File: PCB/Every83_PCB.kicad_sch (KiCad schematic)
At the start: 31 parts, among them J1 781710004, J3 SM03B-SRSS-TB, J4 SM03B-SRSS-TB, Q3 DMG2305, SW101 KMR2, SW102 KMR2, U1 Core52840, U2 AP2112(3.3V), U3 MCP73831T-2ACI/OT, X3 JSTPH

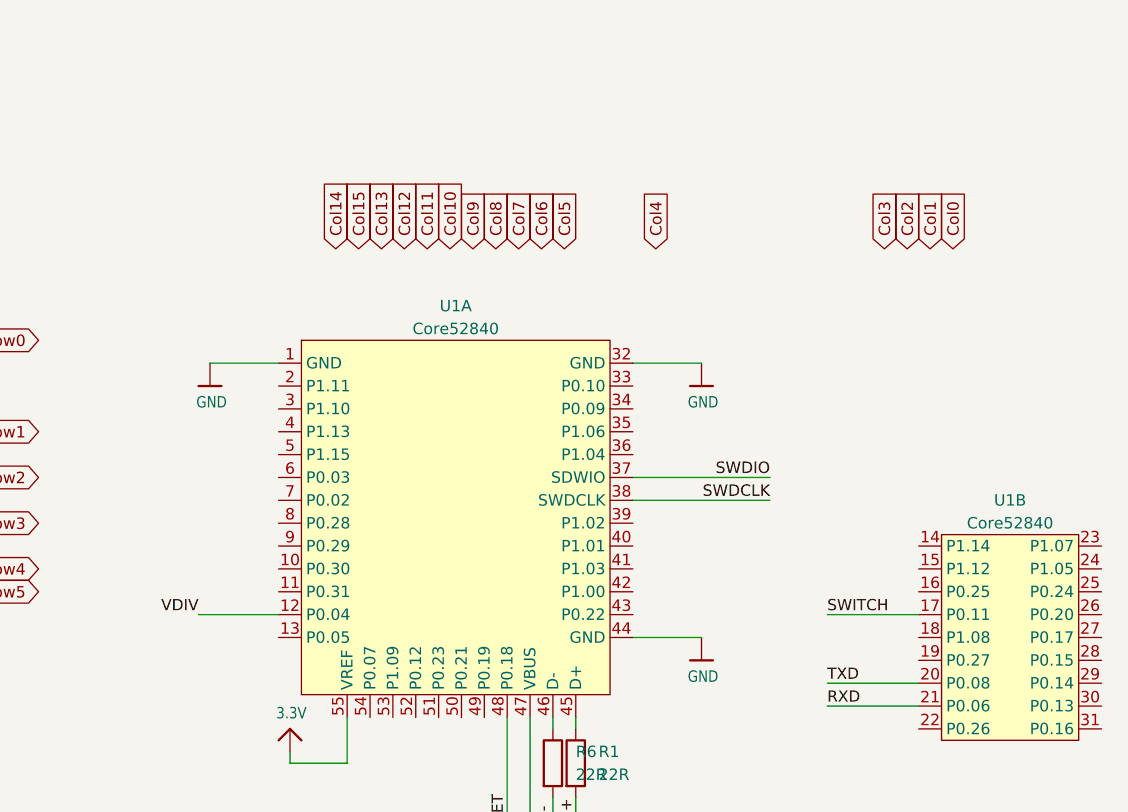
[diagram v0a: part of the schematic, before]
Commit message: More work done
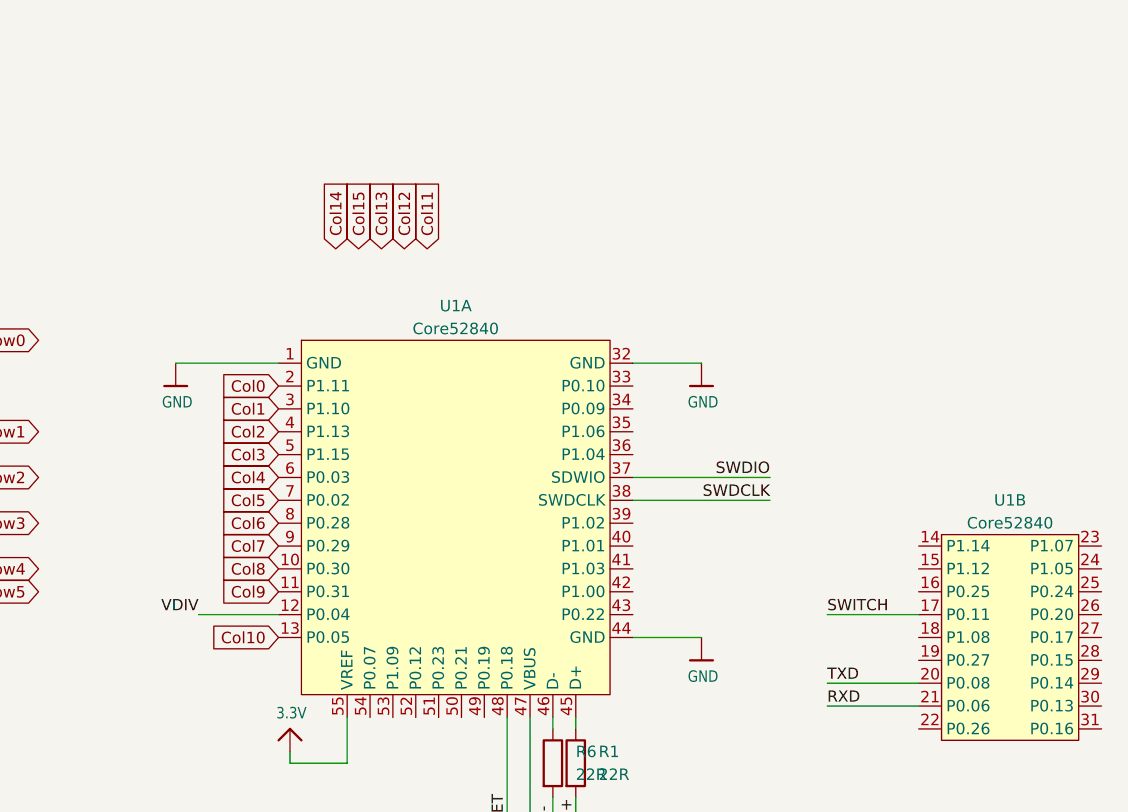
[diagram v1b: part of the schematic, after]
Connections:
- net Col0: now also U1.2 (P1.11)
- net Col1: now also U1.3 (P1.10)
- net Col10: now also U1.13 (P0.05)
- net Col2: now also U1.4 (P1.13)
- net Col3: now also U1.5 (P1.15)
- net Col4: now also U1.6 (P0.03)
- net Col5: now also U1.7 (P0.02)
- net Col6: now also U1.8 (P0.28)
- net Col7: now also U1.9 (P0.29)
- net Col8: now also U1.10 (P0.30)
- net Col9: now also U1.11 (P0.31)
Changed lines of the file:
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@@
 	(wire
 		(pts
-			(xy 120.65 81.28) (xy 128.27 81.28)
+			(xy 116.84 81.28) (xy 128.27 81.28)
 		)
 		(stroke
@@
 	(global_label "Col10"
 		(shape input)
-		(at 147.32 68.58 90)
+		(at 128.27 111.76 180)
 		(fields_autoplaced yes)
 		(effects
@@
 				(size 1.27 1.27)
 			)
-			(justify left)
+			(justify right)
 		)
 		(property "Intersheetrefs" "${INTERSHEET_REFS}"
-			(at 147.32 60.171 90)
+			(at 119.7816 111.76 0)
 			(effects
 				(font
 					(size 1.27 1.27)
 				)
-				(justify left)
+				(justify right)
 				(hide yes)
 			)
@@
 	(global_label "Col8"
 		(shape input)
-		(at 152.4 68.58 90)
+		(at 128.27 104.14 180)
 		(fields_autoplaced yes)
 		(effects
@@
 				(size 1.27 1.27)
 			)
-			(justify left)
+			(justify right)
 		)
 		(property "Intersheetrefs" "${INTERSHEET_REFS}"
-			(at 152.4 61.3011 90)
+			(at 120.9911 104.14 0)
 			(effects
 				(font
 					(size 1.27 1.27)
 				)
-				(justify left)
+				(justify right)
 				(hide yes)
 			)
@@
 	(global_label "Col5"
 		(shape input)
-		(at 160.02 68.58 90)
+		(at 128.27 96.52 180)
 		(fields_autoplaced yes)
 		(effects
@@
 				(size 1.27 1.27)
 			)
-			(justify left)
+			(justify right)
 		)
 		(property "Intersheetrefs" "${INTERSHEET_REFS}"
-			(at 160.02 61.3011 90)
+			(at 120.9911 96.52 0)
 			(effects
 				(font
 					(size 1.27 1.27)
 				)
-				(justify left)
+				(justify right)
 				(hide yes)
 			)
@@
 	(global_label "Col7"
 		(shape input)
-		(at 154.94 68.58 90)
+		(at 128.27 101.6 180)
 		(fields_autoplaced yes)
 		(effects
@@
 				(size 1.27 1.27)
 			)
-			(justify left)
+			(justify right)
 		)
 		(property "Intersheetrefs" "${INTERSHEET_REFS}"
-			(at 154.94 61.3011 90)
+			(at 120.9911 101.6 0)
 			(effects
 				(font
 					(size 1.27 1.27)
 				)
-				(justify left)
+				(justify right)
 				(hide yes)
 			)
@@
 	(global_label "Col9"
 		(shape input)
-		(at 149.86 68.58 90)
+		(at 128.27 106.68 180)
 		(fields_autoplaced yes)
 		(effects
@@
 				(size 1.27 1.27)
 			)
-			(justify left)
+			(justify right)
 		)
 		(property "Intersheetrefs" "${INTERSHEET_REFS}"
-			(at 149.86 61.3805 90)
+			(at 120.9911 106.68 0)
 			(effects
 				(font
 					(size 1.27 1.27)
 				)
-				(justify left)
+				(justify right)
 				(hide yes)
 			)
@@
 	(global_label "Col6"
 		(shape input)
-		(at 157.48 68.58 90)
+		(at 128.27 99.06 180)
 		(fields_autoplaced yes)
 		(effects
@@
 				(size 1.27 1.27)
 			)
-			(justify left)
+			(justify right)
 		)
 		(property "Intersheetrefs" "${INTERSHEET_REFS}"
-			(at 157.48 61.3011 90)
+			(at 120.9911 99.06 0)
 			(effects
 				(font
 					(size 1.27 1.27)
 				)
-				(justify left)
+				(justify right)
 				(hide yes)
 			)
@@
 	(global_label "Col2"
 		(shape input)
-		(at 198.12 68.58 90)
+		(at 128.27 88.9 180)
 		(fields_autoplaced yes)
 		(effects
@@
 				(size 1.27 1.27)
 			)
-			(justify left)
+			(justify right)
 		)
 		(property "Intersheetrefs" "${INTERSHEET_REFS}"
-			(at 198.12 61.3011 90)
+			(at 120.9911 88.9 0)
 			(effects
 				(font
 					(size 1.27 1.27)
 				)
-				(justify left)
+				(justify right)
 				(hide yes)
 			)
@@
 	(global_label "Col3"
 		(shape input)
-		(at 195.58 68.58 90)
+		(at 128.27 91.44 180)
 		(fields_autoplaced yes)
 		(effects
@@
 				(size 1.27 1.27)
 			)
-			(justify left)
+			(justify right)
 		)
 		(property "Intersheetrefs" "${INTERSHEET_REFS}"
-			(at 195.58 61.3011 90)
+			(at 120.9911 91.44 0)
 			(effects
 				(font
 					(size 1.27 1.27)
 				)
-				(justify left)
+				(justify right)
 				(hide yes)
 			)
@@
 	(global_label "Col1"
 		(shape input)
-		(at 200.66 68.58 90)
+		(at 128.27 86.36 180)
 		(fields_autoplaced yes)
 		(effects
@@
 				(size 1.27 1.27)
 			)
-			(justify left)
+			(justify right)
 		)
 		(property "Intersheetrefs" "${INTERSHEET_REFS}"
-			(at 200.66 61.3011 90)
+			(at 120.9911 86.36 0)
 			(effects
 				(font
 					(size 1.27 1.27)
 				)
-				(justify left)
+				(justify right)
 				(hide yes)
 			)
@@
 	(global_label "Col0"
 		(shape input)
-		(at 203.2 68.58 90)
+		(at 128.27 83.82 180)
 		(fields_autoplaced yes)
 		(effects
@@
 				(size 1.27 1.27)
 			)
-			(justify left)
+			(justify right)
 		)
 		(property "Intersheetrefs" "${INTERSHEET_REFS}"
-			(at 203.2 61.3011 90)
+			(at 120.9911 83.82 0)
 			(effects
 				(font
 					(size 1.27 1.27)
 				)
-				(justify left)
+				(justify right)
 				(hide yes)
 			)
@@
 	(global_label "Col4"
 		(shape input)
-		(at 170.18 68.58 90)
+		(at 128.27 93.98 180)
 		(fields_autoplaced yes)
 		(effects
@@
 				(size 1.27 1.27)
 			)
-			(justify left)
+			(justify right)
 		)
 		(property "Intersheetrefs" "${INTERSHEET_REFS}"
-			(at 170.18 61.3011 90)
+			(at 120.9911 93.98 0)
 			(effects
 				(font
 					(size 1.27 1.27)
 				)
-				(justify left)
+				(justify right)
 				(hide yes)
 			)
@@
 	(symbol
 		(lib_id "Adafruit nRF52840 Bluefruit Feather Express Rev D-eagle-import:GND")
-		(at 120.65 83.82 0)
+		(at 116.84 83.82 0)
 		(unit 1)
 		(exclude_from_sim no)
@@
 		(dnp no)
 		(property "Reference" "#U$048"
-			(at 120.65 83.82 0)
+			(at 116.84 83.82 0)
 			(effects
 				(font
@@
 		)
 		(property "Value" "GND"
-			(at 119.126 86.36 0)
+			(at 115.316 86.36 0)
 			(effects
 				(font
@@
 		)
 		(property "Footprint" ""
-			(at 120.65 83.82 0)
+			(at 116.84 83.82 0)
 			(effects
 				(font
@@
 		)
 		(property "Datasheet" ""
-			(at 120.65 83.82 0)
+			(at 116.84 83.82 0)
 			(effects
 				(font
@@
 		)
 		(property "Description" ""
-			(at 120.65 83.82 0)
+			(at 116.84 83.82 0)
 			(effects
 				(font

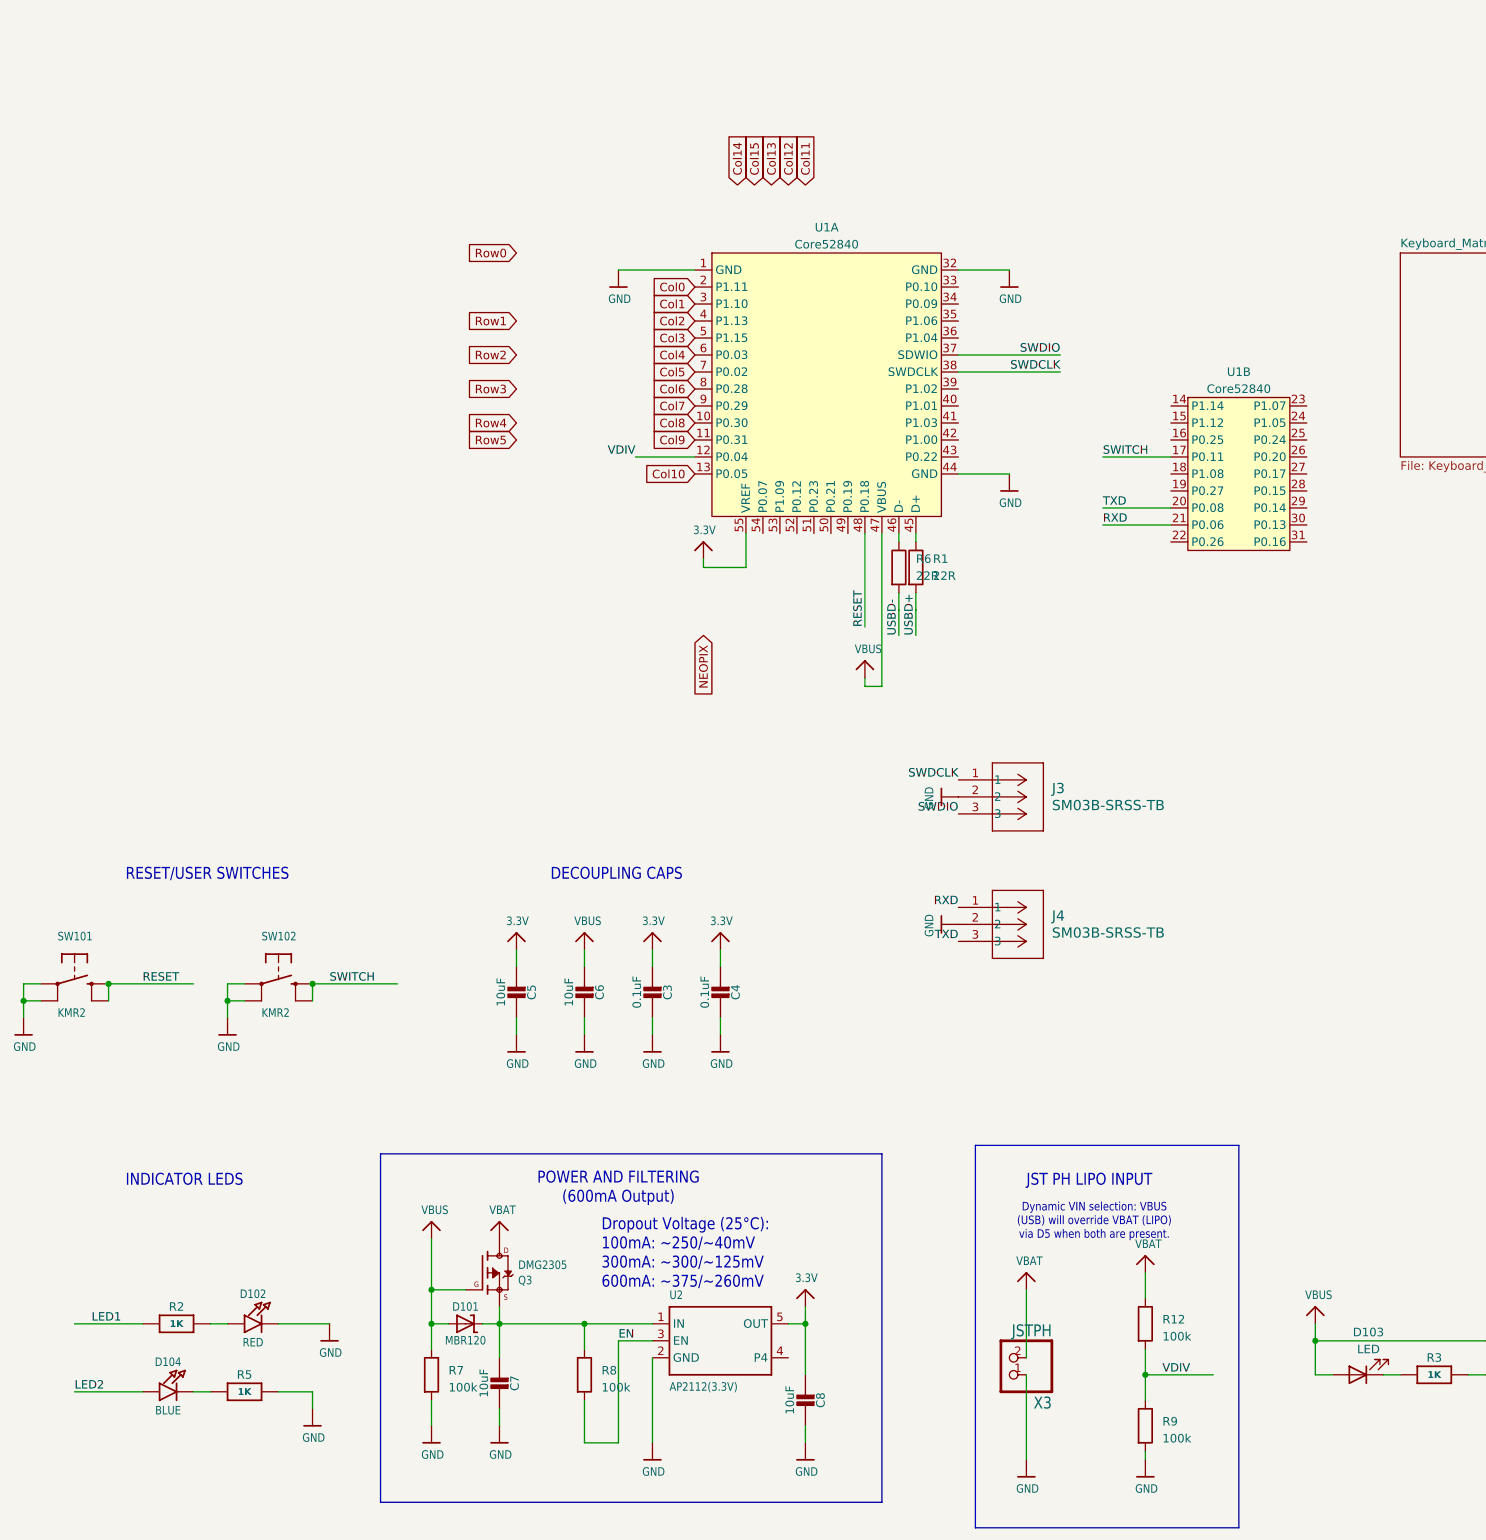
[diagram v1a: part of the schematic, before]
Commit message: Just need to run DRC now
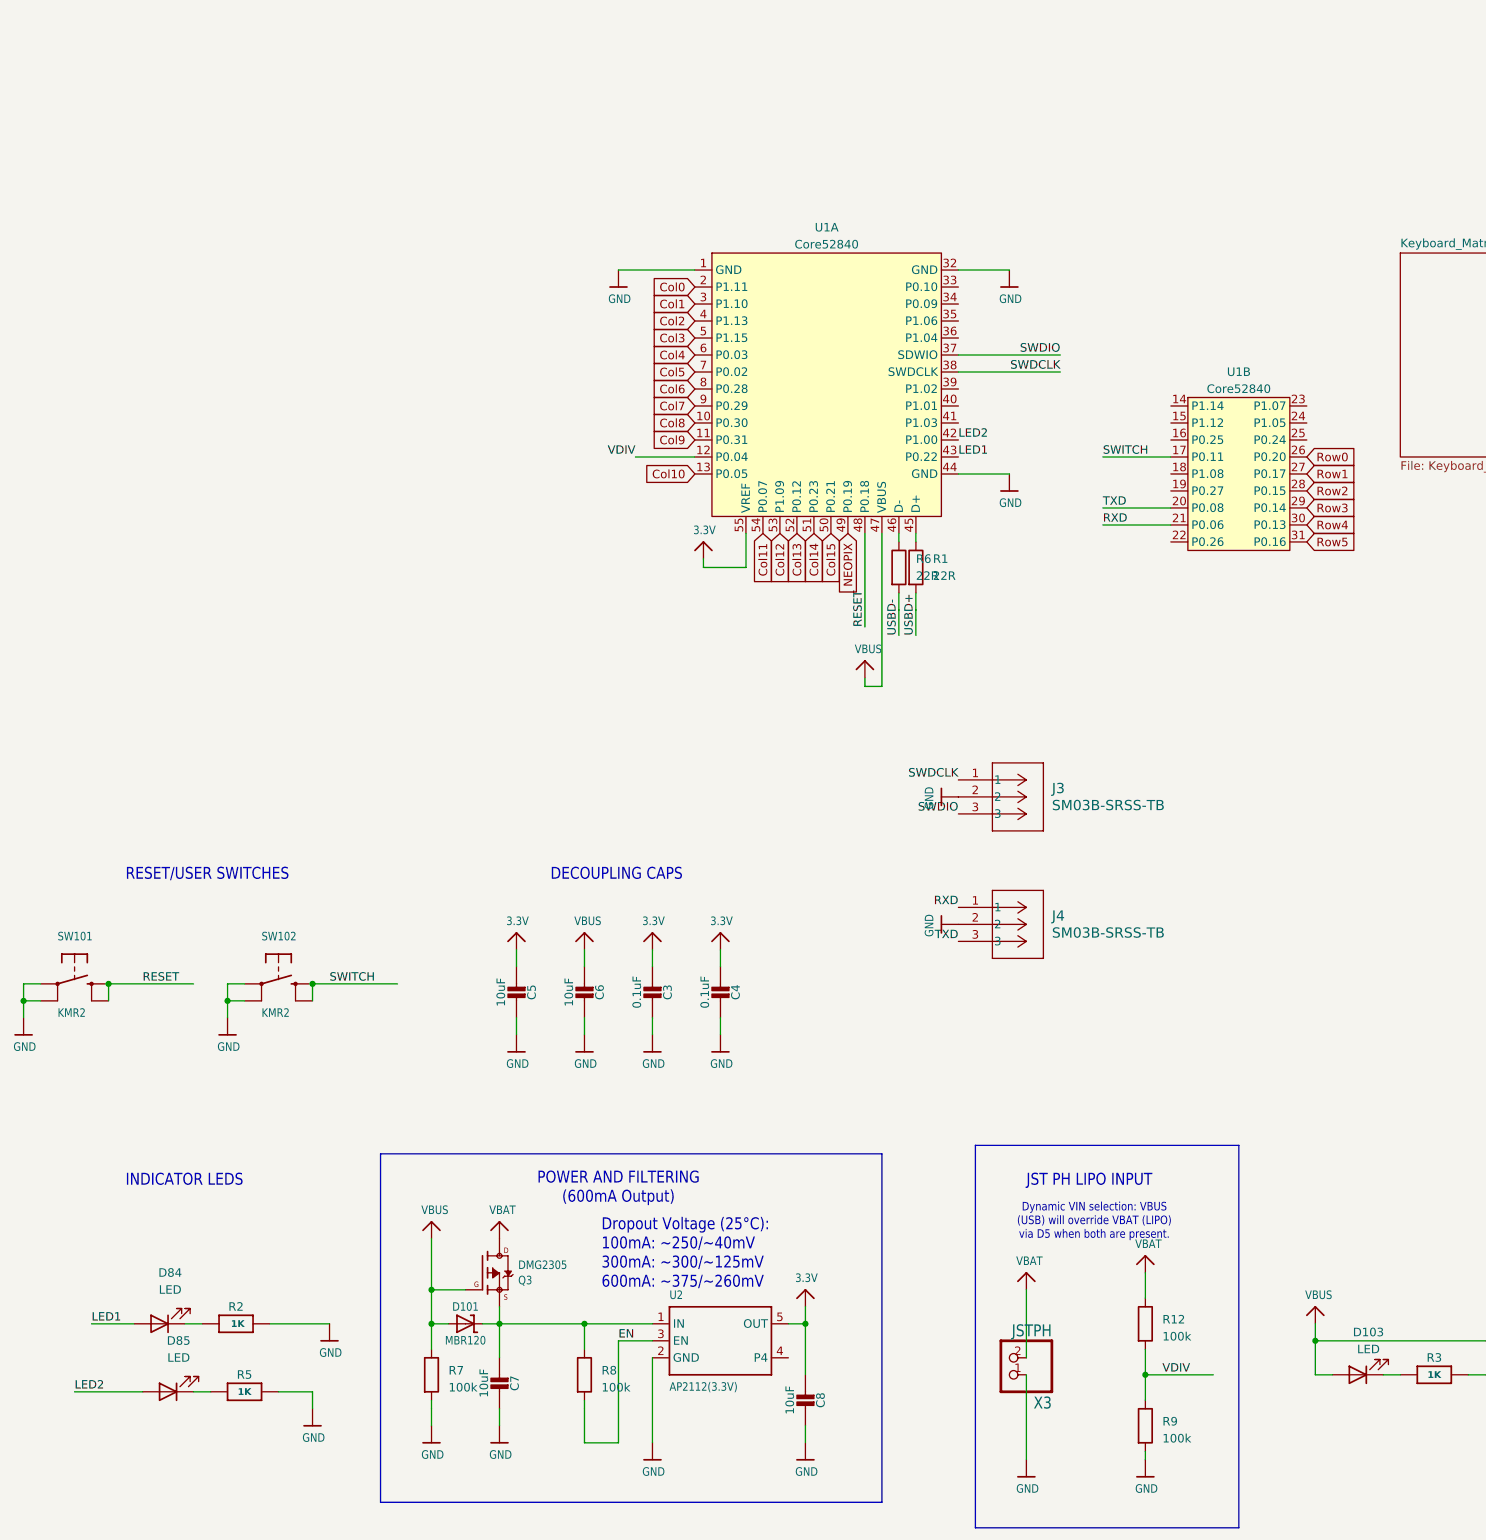
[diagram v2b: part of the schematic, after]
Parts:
- removed D102: RED, Adafruit nRF52840 Bluefruit Feather Express Rev D:CHIPLED_0805_NOOUTLINE, symbol Adafruit nRF52840 Bluefruit Feather Express Rev D-eagle-import:LED0805_NOOUTLINE
- removed D104: BLUE, Adafruit nRF52840 Bluefruit Feather Express Rev D:CHIPLED_0805_NOOUTLINE, symbol Adafruit nRF52840 Bluefruit Feather Express Rev D-eagle-import:LED0805_NOOUTLINE
- added D84, D85: LED, LED_SMD:LED_0805_2012Metric, symbol Device:LED
- R2, R3, R5: footprint Adafruit nRF52840 Bluefruit Feather Express Rev D:0603-NO -> Resistor_SMD:R_0603_1608Metric
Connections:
- net Col11: now also U1.54 (P0.07)
- net Col12: now also U1.53 (P1.09)
- net Col13: now also U1.52 (P0.12)
- net Col14: now also U1.51 (P0.23)
- net Col15: now also U1.50 (P0.21)
- net GND: now also R2.2
- net LED1: now also U1.43 (P0.22), D84.2 (A); no longer R2.1
- net LED2: now also U1.42 (P1.00), D85.2 (A)
- net NEOPIX: now also U1.49 (P0.19)
- net Row0: now also U1.26 (P0.20)
- net Row1: now also U1.27 (P0.17)
- net Row2: now also U1.28 (P0.15)
- net Row3: now also U1.29 (P0.14)
- net Row4: now also U1.30 (P0.13)
- net Row5: now also U1.31 (P0.16)
- net at R5.1: now also D85.1 (K)
- new net: D84.1 (K), R2.1
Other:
- moved on the sheet: R2
